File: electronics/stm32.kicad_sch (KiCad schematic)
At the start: 38 parts, among them J1 USB_B_Micro, J2 Conn_ARM_JTAG_SWD_10, SW1 PTS645SK50SMTR92LFS, U1 USBLC6-2SC6, U2 STM32F446RETx, Y1 Crystal_GND24

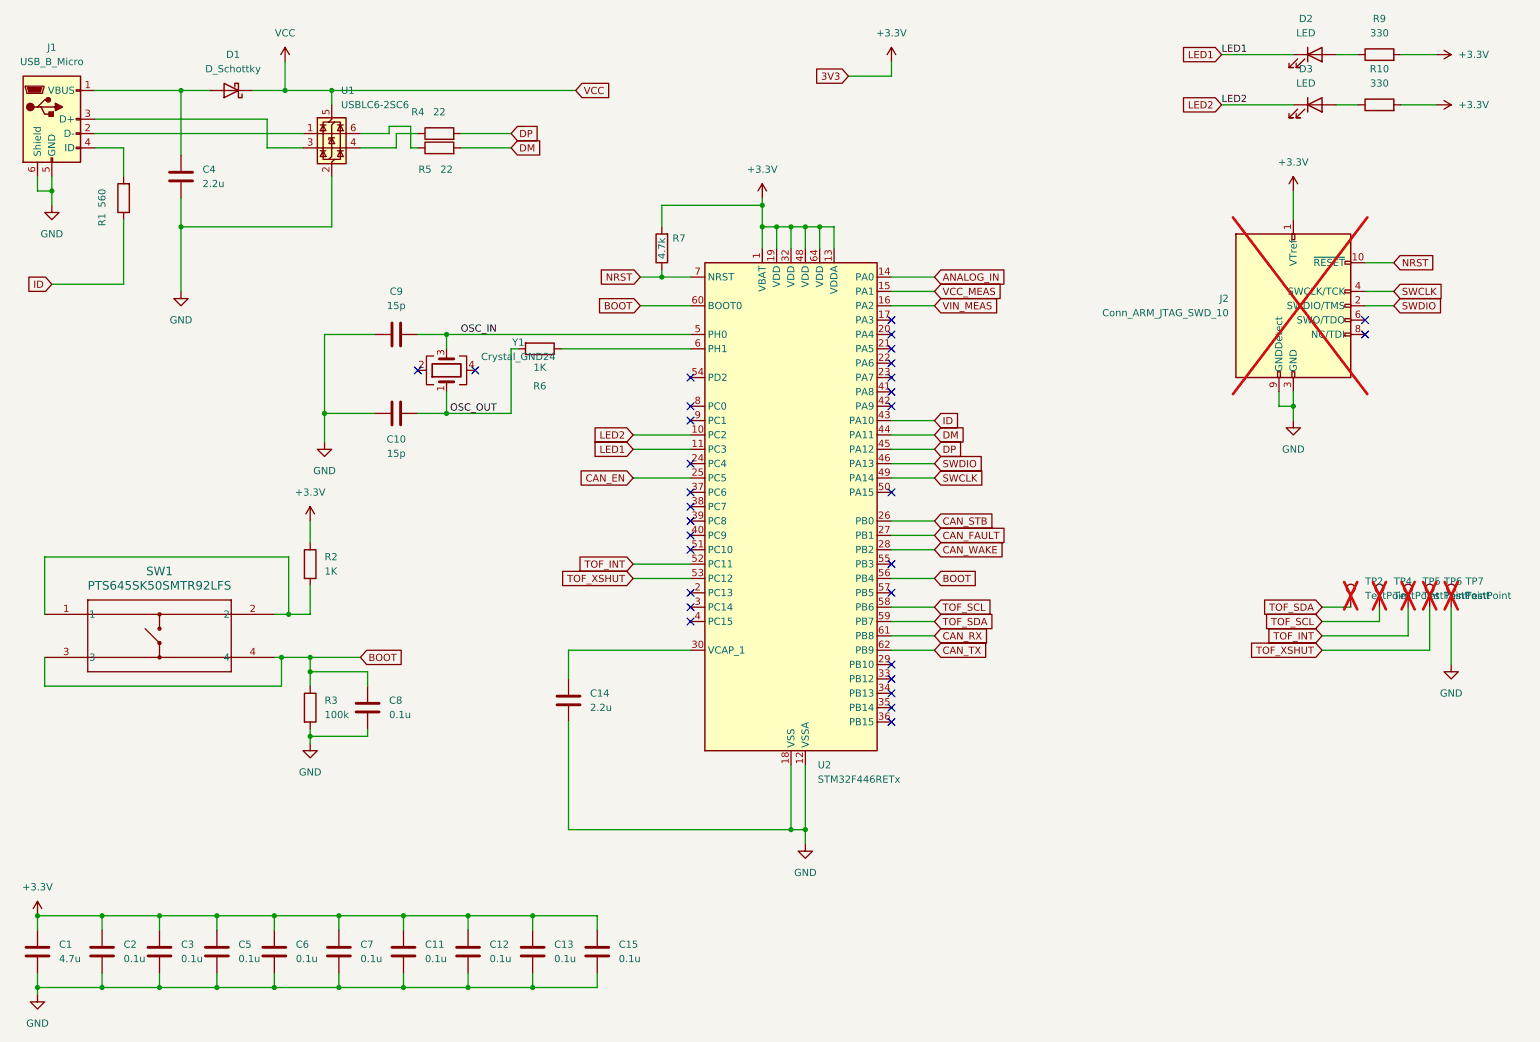
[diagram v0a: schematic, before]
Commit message: Ordered this version.
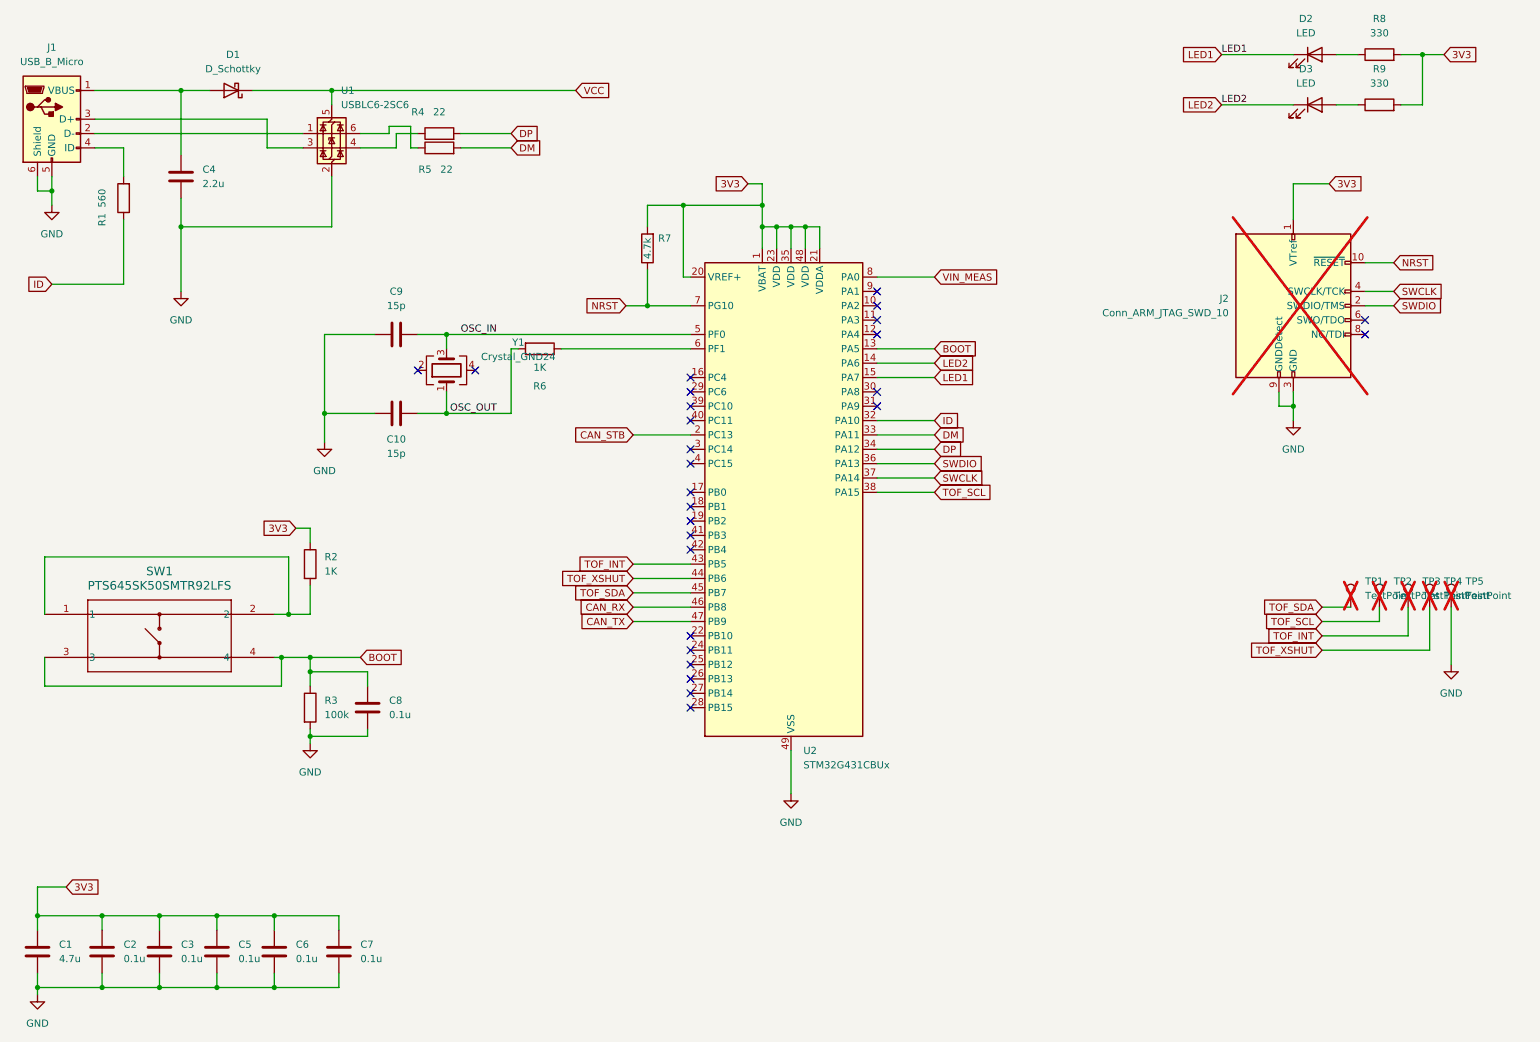
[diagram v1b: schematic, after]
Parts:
- removed C11, C12, C13, C15: 0.1u, Capacitor_SMD:C_0402_1005Metric, symbol Device:C
- removed C14: 2.2u, Capacitor_SMD:C_0603_1608Metric, symbol Device:C
- removed U2: STM32F446RETx, Package_QFP:LQFP-64_10x10mm_P0.5mm, symbol MCU_ST_STM32F4:STM32F446RETx
- added U2: STM32G431CBUx, Package_DFN_QFN:QFN-48-1EP_7x7mm_P0.5mm_EP5.6x5.6mm, symbol MCU_ST_STM32G4:STM32G431CBUx
- C1: footprint Capacitor_SMD:C_0805_2012Metric -> Capacitor_SMD:C_0603_1608Metric; JLCPCB (none) -> C1705
- R1: footprint Resistor_SMD:R_0603_1608Metric -> Resistor_SMD:R_0402_1005Metric; JLCPCB (none) -> C25126
- R2, R6: JLCPCB (none) -> C11702
- renumbered R9 to R8, R10 to R9, TP2 to TP1, TP4 to TP2, TP5 to TP3, TP6 to TP4, TP7 to TP5
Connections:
- net BOOT: now also U2.13 (PA5)
- net CAN_RX: now also U2.46 (PB8)
- net CAN_STB: now also U2.2 (PC13)
- net CAN_TX: now also U2.47 (PB9)
- net DM: now also U2.33 (PA11)
- net DP: now also U2.34 (PA12)
- net GND: now also U2.49 (VSS)
- net ID: now also U2.32 (PA10)
- net LED1: now also U2.15 (PA7)
- net LED2: now also U2.14 (PA6)
- net NRST: now also U2.7 (PG10)
- net OSC_IN: now also U2.5 (PF0)
- net SWCLK: now also U2.37 (PA14)
- net SWDIO: now also U2.36 (PA13)
- net TOF_INT: now also U2.43 (PB5)
- net TOF_SCL: now also U2.38 (PA15)
- net TOF_SDA: now also U2.45 (PB7)
- net TOF_XSHUT: now also U2.44 (PB6)
- net VIN_MEAS: now also U2.8 (PA0)
- net at R6.1: now also U2.6 (PF1)
- net +3.3V renamed 3V3
- net 3V3: now also U2.1 (VBAT), U2.20 (VREF+), U2.21 (VDDA), U2.23 (VDD), U2.35 (VDD), U2.48 (VDD)
- no-connect marks 31 -> 27
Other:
- moved on the sheet: R7
